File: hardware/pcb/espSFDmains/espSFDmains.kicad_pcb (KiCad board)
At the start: 2 copper layers, 130.2 x 61 mm, 36 parts, among them J1 Mains, J2 Mains Motor, J3 VDD, J4 VDD, J5 Motor, J6 Motor, J7 Conn_02x10_Odd_Even, J8 Conn_02x10_Odd_Even, J9 Conn_02x10_Odd_Even, Q1 2N7002E, Q2 2N7002H, U2 LM2675N-5, U3 WEMOS_D1_mini

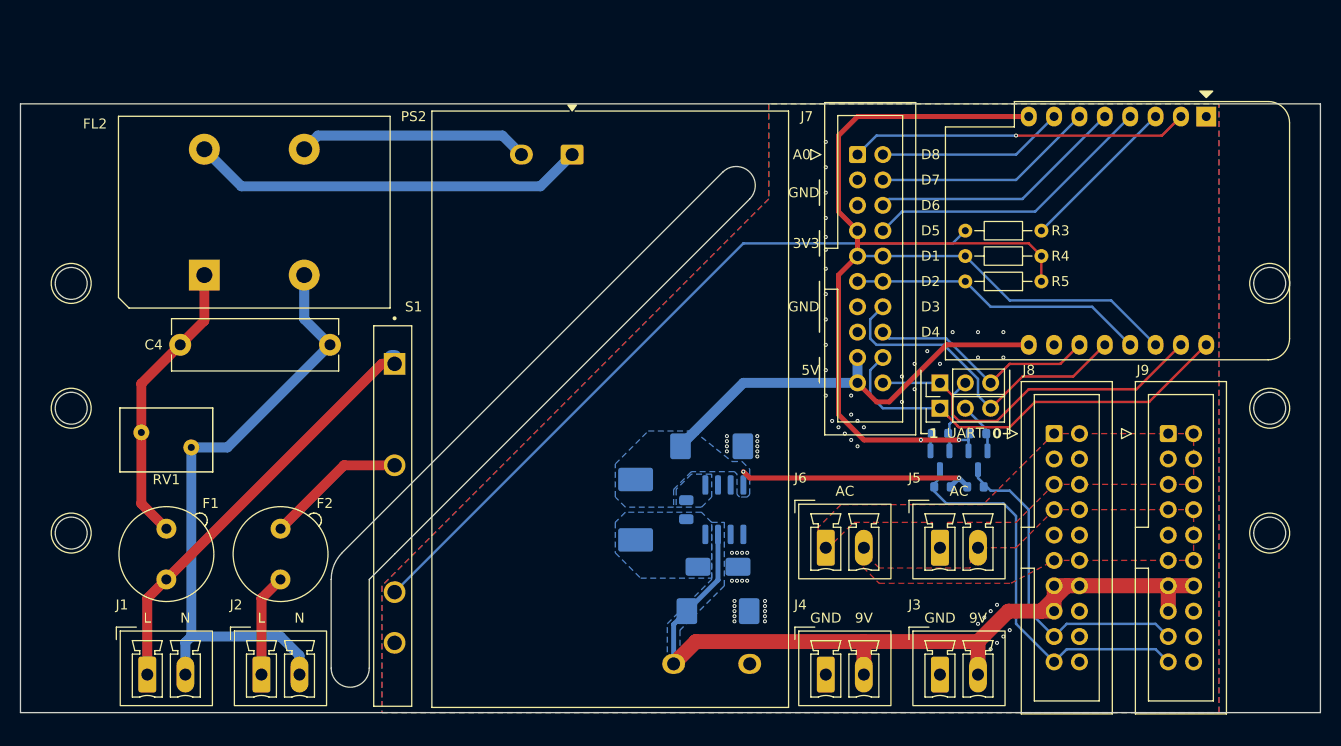
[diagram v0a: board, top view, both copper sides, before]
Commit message: jfgj
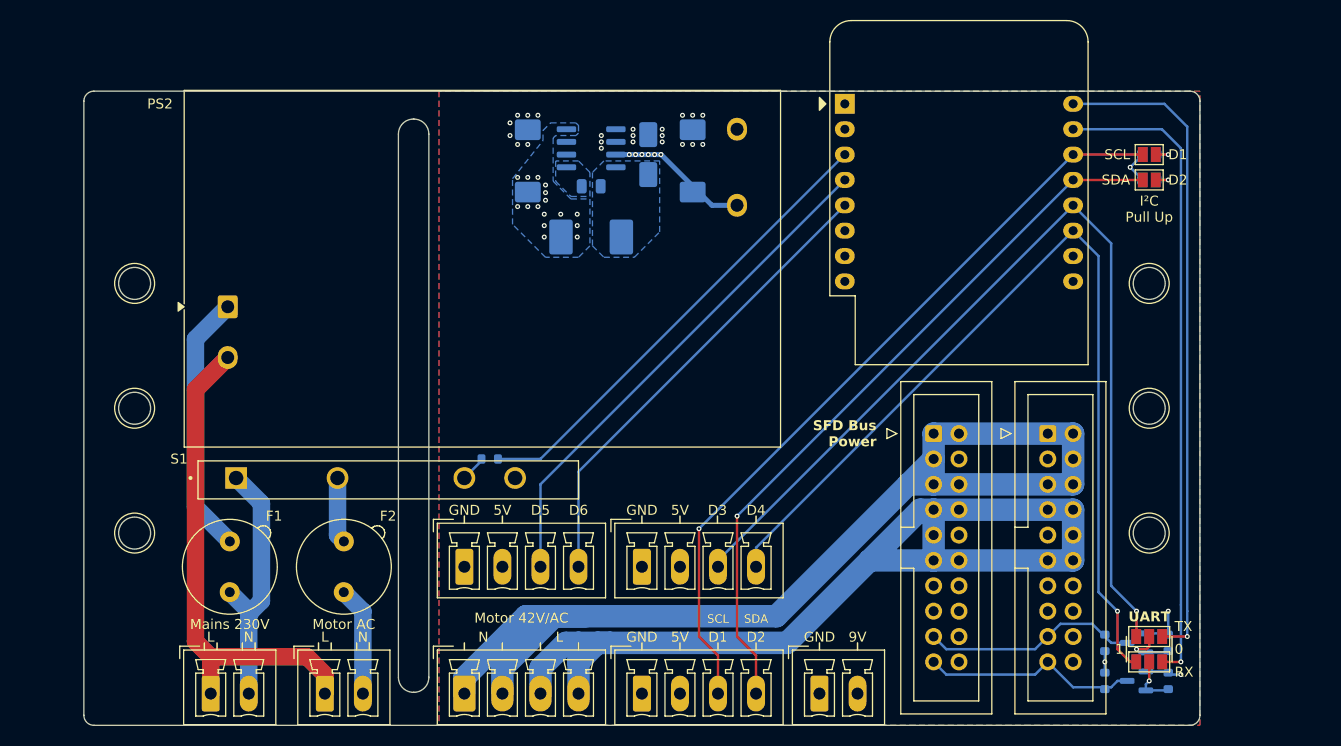
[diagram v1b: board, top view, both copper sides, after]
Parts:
- removed C4: 0.1uF/275Vac, Capacitor_THT:C_Rect_L16.5mm_W5.0mm_P15.00mm_MKT
- removed FL2: Choke_CommonMode_PulseElectronics_PH9455x156NL, Inductor_THT:L_CommonMode_PulseElectronics_PH9455xxx6NL_2
- removed J6: Motor, Connector_Phoenix_MC:PhoenixContact_MCV_1,5_2-G-3.81_1x02_P3.81mm_Vertical
- removed J7: Conn_02x10_Odd_Even, Connector_IDC:IDC-Header_2x10_P2.54mm_Vertical
- removed RV1: 10D561K, Varistor:RV_Disc_D9mm_W6.1mm_P5mm
- added J10: Conn_01x04_Socket, Connector_Phoenix_MC:PhoenixContact_MCV_1,5_4-G-3.81_1x04_P3.81mm_Vertical, F.Cu at (93.0, 152.1)
- added J11: Conn_01x04_Socket, Connector_Phoenix_MC:PhoenixContact_MCV_1,5_4-G-3.81_1x04_P3.81mm_Vertical, F.Cu at (93.0, 139.4)
- added JP3: SolderJumper_2_Open, Jumper:SolderJumper-2_P1.3mm_Open_Pad1.0x1.5mm, F.Cu at (143.8, 98.1)
- added JP4: SolderJumper_2_Open, Jumper:SolderJumper-2_P1.3mm_Open_Pad1.0x1.5mm, F.Cu at (143.8, 100.6)
- J4: value VDD -> Conn_01x04_Socket; footprint Connector_Phoenix_MC:PhoenixContact_MCV_1,5_2-G-3.81_1x02_P3.81mm_Vertical -> Connector_Phoenix_MC:PhoenixContact_MCV_1,5_4-G-3.81_1x04_P3.81mm_Vertical
- J5: footprint Connector_Phoenix_MC:PhoenixContact_MCV_1,5_2-G-3.81_1x02_P3.81mm_Vertical -> Connector_Phoenix_MC:PhoenixContact_MCV_1,5_4-G-3.81_1x04_P3.81mm_Vertical
- JP1, JP2: footprint Connector_PinHeader_2.54mm:PinHeader_1x03_P2.54mm_Vertical -> Jumper:SolderJumper-3_P1.3mm_Open_Pad1.0x1.5mm
- R3, R4, R5: footprint Resistor_THT:R_Axial_DIN0204_L3.6mm_D1.6mm_P7.62mm_Horizontal -> Resistor_SMD:R_0603_1608Metric; moved to B.Cu
- moved R3 59.8 mm to (77.8, 128.6)
- moved J5 49.8 mm to (75.2, 152.1)
- moved C1 45.2 mm to (98.1, 98.7), turned to 90 degrees
- moved D1 41.9 mm to (93.7, 98.1), turned to 90 degrees
- moved U2 38.6 mm to (87.9, 97.5), turned to 0 degrees
- moved J4 37.8 mm to (75.2, 139.4)
- moved PS2 37.7 mm to (51.5, 113.3), turned to 0 degrees
- moved U3 36.2 mm to (113.3, 93.0), turned to 0 degrees
- moved JP1 34.9 mm to (143.8, 148.9), turned to 180 degrees
- moved C3 34.0 mm to (81.6, 98.7), turned to 90 degrees
- moved C2 33.8 mm to (87.9, 101.3), turned to 0 degrees
- moved R1 33.7 mm to (145.7, 150.8), turned to 90 degrees
- moved JP2 31.0 mm to (143.8, 146.4), turned to 180 degrees
- moved Q1 29.6 mm to (142.6, 150.8), turned to 180 degrees
- moved R2 28.3 mm to (145.7, 147.0), turned to 90 degrees
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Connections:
- F1 pad 2: Net-(C4-Pad1) -> Net-(PS2-AC/L)
- J1 pad 1: LINE -> NEUT
- J1 pad 2: NEUT -> LINE
- J2 pad 1: 230V Motor -> NEUT
- J2 pad 2: NEUT -> 230V Motor
- J4 pad 2: VDD -> VCC
- J5 pad 2: Motor L -> Motor N
- PS2 pad 2: Net-(PS2-AC/N) -> NEUT
- R4 pad 2: D1/SCL -> Net-(JP3-A)
- R5 pad 2: D2/SDA -> Net-(JP4-A)
- U3 pad 2: A0 -> unconnected-(U3-A0-Pad2)
- U3 pad 6: D7 -> unconnected-(U3-MOSI/D7-Pad6)
- U3 pad 7: D8 -> unconnected-(U3-CS/D8-Pad7)
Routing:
- net Motor N: track 0.00 -> 111.4 mm
- net Motor L: track 0.00 -> 102.0 mm
- net +3.3V: track 89.4 -> 11.7 mm, vias 2 -> 3
- net VDD: track 84.3 -> 14.2 mm, vias 0 -> 6
- net Net-(S1-+LED): track 72.1 -> 2.62 mm
- net D4/RX1: track 23.6 -> 93.0 mm, vias 0 -> 1
- net VCC: track 67.6 -> 2.16 mm, vias 2 -> 17
- net D3/TX1: track 34.2 -> 96.8 mm, vias 0 -> 1
- net D1/SCL: track 33.5 -> 77.3 mm, vias 0 -> 1
- net D2/SDA: track 29.9 -> 73.1 mm, vias 0 -> 1
- net A0: track 34.0 -> 0.00 mm, vias 1 -> 0
- net En Motor: track 16.2 -> 47.4 mm
- net RX/RX0: track 35.7 -> 64.9 mm, vias 0 -> 1
- net Net-(C4-Pad1): track 29.1 -> 0.00 mm
- net TX/TX0: track 42.7 -> 65.9 mm, vias 0 -> 1
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- added copper zone on In1.Cu, net +3.3V
- added copper zone on B.Cu, net Motor L
- added copper zone on B.Cu, net Motor N
- added copper zone on In2.Cu, net VCC
- added copper zone on In1.Cu, net VDD
- removed copper zone on F.Cu, net Motor L
- removed copper zone on F.Cu, net Motor N
- removed copper zone on B.Cu, net VDD
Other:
- board size 130.2 x 61 mm -> 111.8 x 63.5 mm
- copper layers 2 -> 4
- board text added: "I²C Pull Up"
- board text added: "Mains 230V"
- board text added: "Motor 42V/AC"
- board text added: "Motor AC"
- board text added: "RX"
- board text added: "SCL"
- board text added: "SDA"
- board text added: "SFD Bus Power"
- board text added: "TX"
- board text removed: "3V3"
- board text removed: "A0"
- board text removed: "AC"
- board text removed: "D7"
- board text removed: "D8"
